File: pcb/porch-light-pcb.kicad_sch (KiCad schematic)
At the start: 11 parts, among them J1 1-2834011-3, J2 Conn_01x02, K1 PRY2-3V-450-1A-EF, Q1 PN2222A

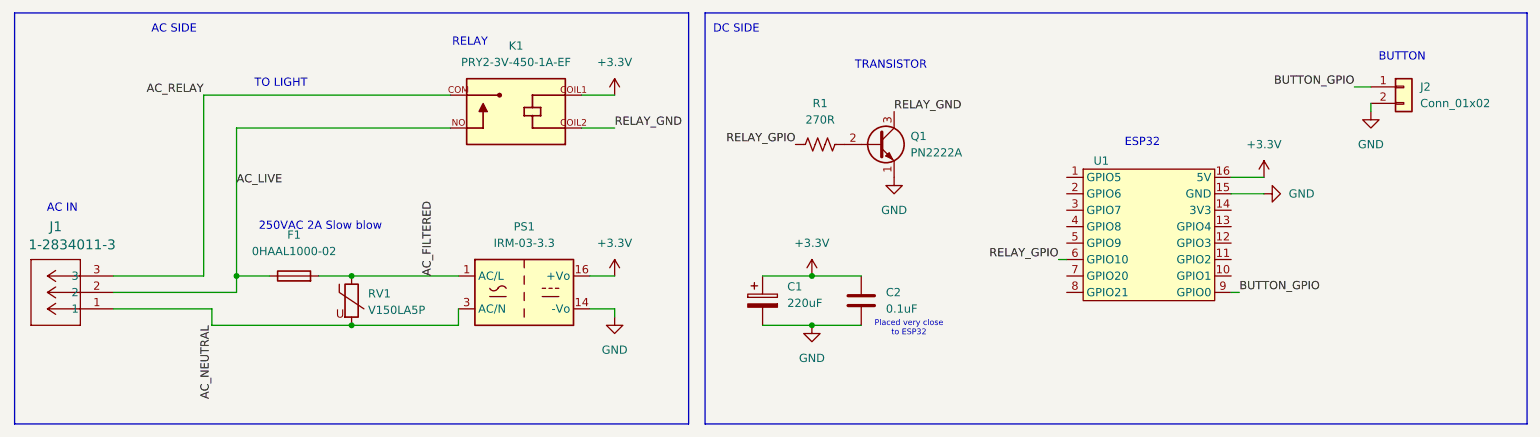
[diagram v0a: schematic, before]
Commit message: updated gitignore
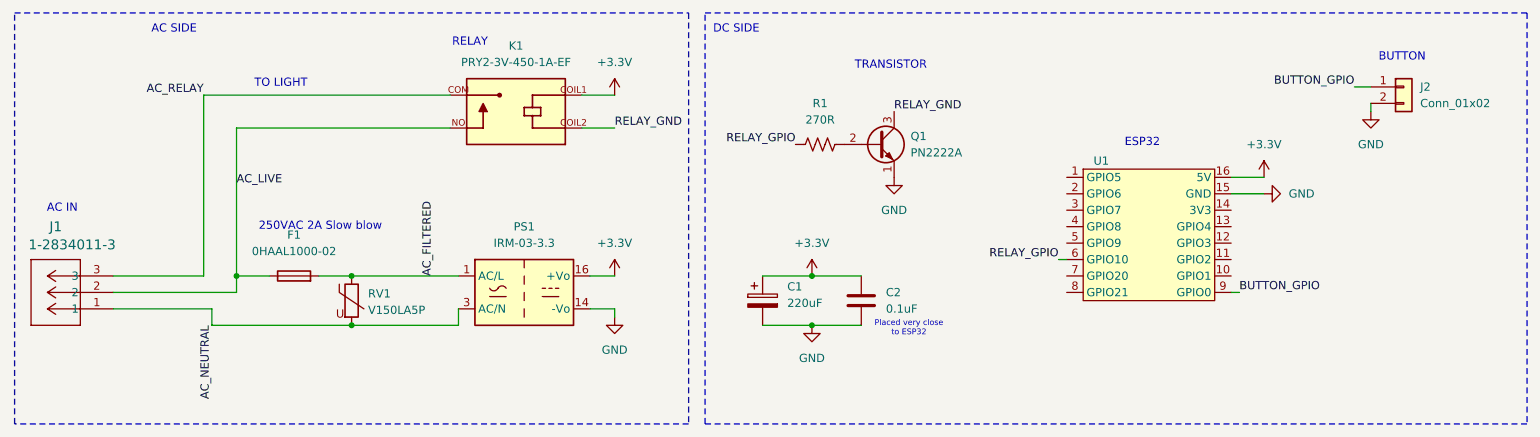
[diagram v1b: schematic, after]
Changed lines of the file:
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@@
 		(stroke
 			(width 0)
-			(type default)
+			(type dash)
 		)
 		(fill
@@
 		(stroke
 			(width 0)
-			(type default)
+			(type dash)
 		)
 		(fill
